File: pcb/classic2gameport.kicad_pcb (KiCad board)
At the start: 2 copper layers, 58 x 45 mm, 39 parts, among them J1 Conn_01x04, J2 Conn_02x05_Odd_Even, J3 DB15_Male, J4 Conn_01x04, Q1 Q_PMOS_GSD, Q2 Q_PMOS_GSD, Q3 Q_PMOS_GSD, Q4 Q_PMOS_GSD, Q5 Q_PMOS_GSD, Q6 Q_PMOS_GSD, Q7 Q_PMOS_GSD, Q8 Q_PMOS_GSD, U1 74HC14, U2 74HC14, U3 LM3480-3.3, U4 STM32F030K6Tx

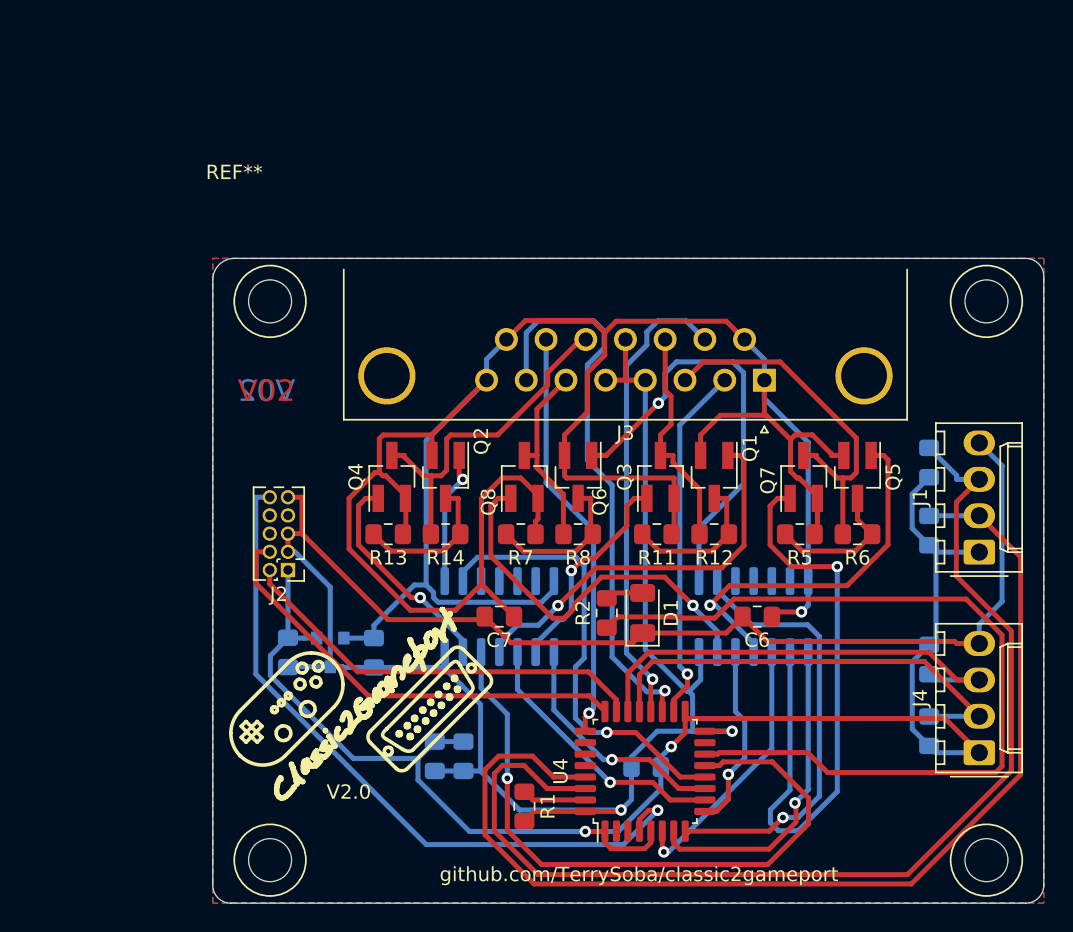
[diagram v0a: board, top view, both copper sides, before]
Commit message: Redesign again
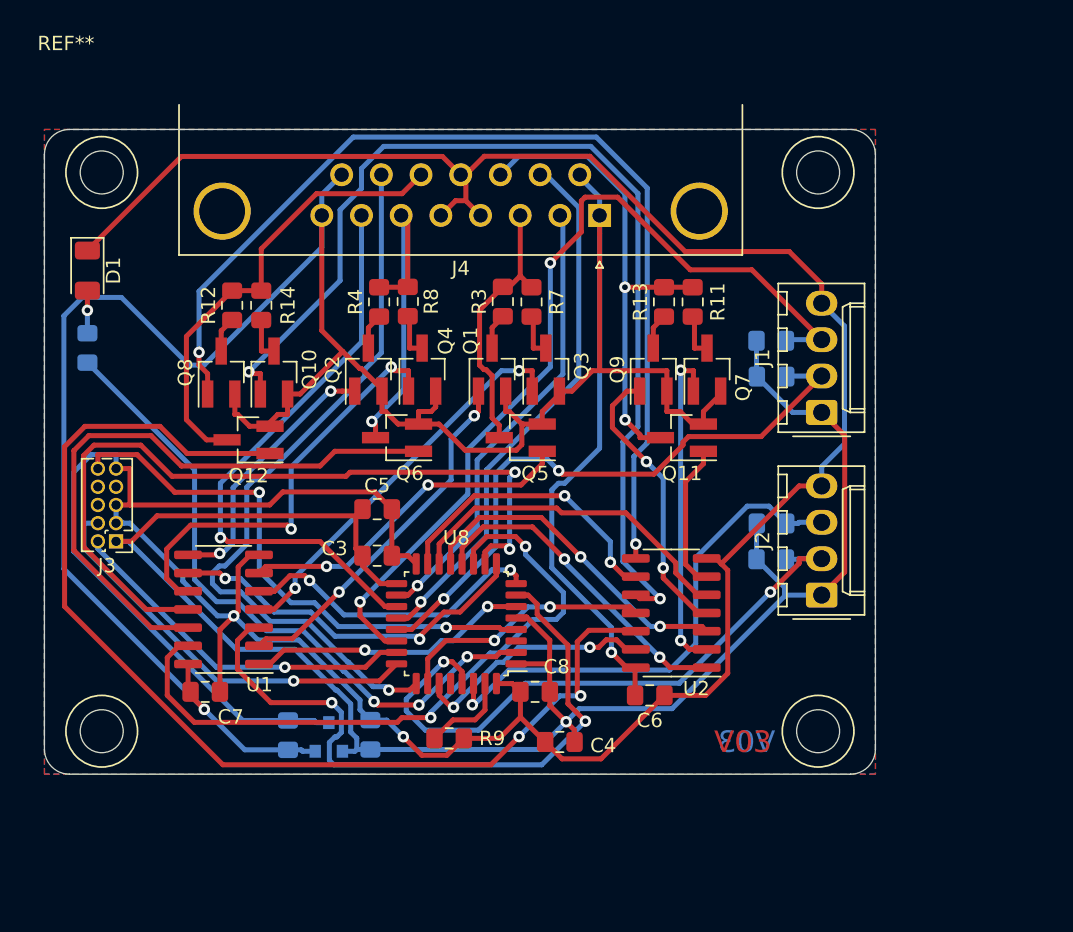
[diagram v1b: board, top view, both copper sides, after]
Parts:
- removed U3: LM3480-3.3, Package_TO_SOT_SMD:SOT-23
- removed U4: STM32F030K6Tx, Package_QFP:LQFP-32_7x7mm_P0.8mm
- added C8: 100nF, Capacitor_SMD:C_0805_2012Metric_Pad1.15x1.40mm_HandSolder, F.Cu at (107.0, 67.8)
- added Q10: Q_PMOS_GSD, Package_TO_SOT_SMD:SOT-23_Handsoldering, F.Cu at (88.8, 45.5)
- added Q11: Q_PMOS_GSD, Package_TO_SOT_SMD:SOT-23_Handsoldering, F.Cu at (117.2, 50.0)
- added Q12: Q_PMOS_GSD, Package_TO_SOT_SMD:SOT-23_Handsoldering, F.Cu at (87.0, 50.2)
- added Q9: Q_PMOS_GSD, Package_TO_SOT_SMD:SOT-23_Handsoldering, F.Cu at (115.2, 45.3)
- added U5: LM3480-3.3, Package_TO_SOT_SMD:SOT-23, B.Cu at (92.6, 70.9)
- added U8: STM32F030K6Tx, Package_QFP:LQFP-32_7x7mm_P0.8mm, F.Cu at (101.5, 63.0)
- C3: value 1µF -> 100nF; moved to F.Cu
- C4: value 4.7µF -> 1µF; moved to F.Cu
- C5: value 100nF -> 4.7µF; moved to F.Cu
- J2: value Conn_02x05_Odd_Even -> Conn_01x04; footprint Connector_PinHeader_1.27mm:PinHeader_2x05_P1.27mm_Vertical -> Connector_Molex:Molex_KK-254_AE-6410-04A_1x04_P2.54mm_Vertical
- J3: value DB15_Male -> Conn_02x05_Odd_Even; footprint Connector_Dsub:DSUB-15_Male_Horizontal_P2.77x2.84mm_EdgePinOffset4.94mm_Housed_MountingHolesOffset7.48mm -> Connector_PinHeader_1.27mm:PinHeader_2x05_P1.27mm_Vertical
- J4: value Conn_01x04 -> DB15_Male; footprint Connector_Molex:Molex_KK-254_AE-6410-04A_1x04_P2.54mm_Vertical -> Connector_Dsub:DSUB-15_Male_Horizontal_P2.77x2.84mm_EdgePinOffset4.94mm_Housed_MountingHolesOffset7.48mm
- R1: value 10k -> 1kR; moved to B.Cu
- R10: value 1kR -> 470R
- R11, R12, R13, R14, R7, R8: value 49k9 -> 100kR
- R2: value 470R -> 1kR; moved to B.Cu
- R3, R4: value 1kR -> 100kR; moved to F.Cu
- R5, R6: value 49k9 -> 1kR; moved to B.Cu
- R9: value 1kR -> 10k; moved to F.Cu
- U1, U2: moved to F.Cu
- moved R10 62.6 mm to (75.8, 43.8), turned to 90 degrees
- moved J3 46.6 mm to (77.8, 57.2)
- moved J4 45.9 mm to (111.5, 34.5), turned to 180 degrees
- moved D1 45.5 mm to (75.8, 38.4), turned to 270 degrees
- moved R4 40.0 mm to (96.1, 40.5)
- moved J2 37.3 mm to (127.0, 61.0), turned to 90 degrees
- moved R12 37.2 mm to (85.9, 40.8), turned to 90 degrees
- moved U1 37.0 mm to (85.2, 62.0), turned to 180 degrees
- moved R1 34.6 mm to (123.5, 45.8), turned to 0 degrees
- moved R3 33.8 mm to (104.7, 40.5)
- moved R9 33.5 mm to (101.0, 71.0), turned to 0 degrees
- moved C5 26.0 mm to (96.0, 55.0), turned to 0 degrees
- moved R13 25.2 mm to (116.0, 40.5), turned to 90 degrees
- moved Q5 23.7 mm to (106.0, 50.0), turned to 180 degrees
- moved Q8 22.4 mm to (85.1, 45.5)
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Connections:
- C1 pad 1: 5V -> 3.3V
- C2 pad 1: 3.3V -> 5V
- J1 pad 2: SCL -> SCL2
- J1 pad 3: SDA -> SDA2
- J2 pad 2: SWDIO -> SCL
- J2 pad 3: GND -> SDA
- J2 pad 4: SWCLK -> GND
- J3 pad 1: 5V -> 3.3V
- J3 pad 10: BUTTON3 -> NRST
- J3 pad 2: BUTTON1 -> SWDIO
- J3 pad 3: JS1_X_AXIS -> GND
- J3 pad 4: GND -> SWCLK
- J3 pad 6: JS1_Y_AXIS -> (no net)
- J3 pad 7: BUTTON2 -> (no net)
- J3 pad 8: 5V -> (no net)
- J3 pad 9: 5V -> GND
- J4 pad 1: 3.3V -> 5V
- J4 pad 2: SCL2 -> BUTTON1
- J4 pad 3: SDA2 -> JS1_X_AXIS
- Q3 pad 3: JS2_X_AXIS -> Net-(Q3-Pad3)
- Q4 pad 3: JS2_Y_AXIS -> Net-(Q4-Pad3)
- Q5 pad 3: Net-(Q5-Pad3) -> JS1_X_AXIS
- Q6 pad 3: Net-(Q6-Pad3) -> JS1_Y_AXIS
- Q7 pad 3: JS1_X_AXIS -> Net-(Q7-Pad3)
- Q8 pad 3: JS1_Y_AXIS -> Net-(Q8-Pad3)
- R1 pad 1: Net-(R1-Pad1) -> 3.3V
- R1 pad 2: GND -> SCL2
- R10 pad 1: 3.3V -> Net-(R10-Pad1)
- R10 pad 2: SDA2 -> Net-(D1-Pad2)
- R11 pad 1: 5V -> Net-(Q7-Pad3)
- R11 pad 2: Net-(Q1-Pad3) -> JS2_X_AXIS
- R12 pad 1: Net-(Q1-Pad3) -> Net-(Q8-Pad3)
- R12 pad 2: JS2_X_AXIS -> JS2_Y_AXIS
- R13 pad 1: 5V -> Net-(Q9-Pad3)
- R13 pad 2: Net-(Q2-Pad3) -> JS2_X_AXIS
- R14 pad 1: Net-(Q2-Pad3) -> Net-(Q10-Pad3)
- R2 pad 1: Net-(R2-Pad1) -> 3.3V
- R2 pad 2: Net-(D1-Pad2) -> SCL
- R3 pad 1: 3.3V -> Net-(Q1-Pad3)
- R3 pad 2: SCL -> JS1_X_AXIS
- R4 pad 1: 3.3V -> Net-(Q2-Pad3)
- R4 pad 2: SDA -> JS1_Y_AXIS
- R5 pad 1: 5V -> 3.3V
- R5 pad 2: Net-(Q5-Pad3) -> SDA2
- R6 pad 1: Net-(Q5-Pad3) -> 3.3V
- R6 pad 2: JS1_X_AXIS -> SDA
- R7 pad 1: 5V -> Net-(Q3-Pad3)
- R7 pad 2: Net-(Q6-Pad3) -> JS1_X_AXIS
- R8 pad 1: Net-(Q6-Pad3) -> Net-(Q4-Pad3)
- R9 pad 1: 3.3V -> Net-(R9-Pad1)
- R9 pad 2: SCL2 -> GND
- U1 pad 1: JS1_X2 -> JS1_X1
- U1 pad 10: (no net) -> Net-(Q4-Pad1)
- U1 pad 11: (no net) -> JS1_Y2
- U1 pad 12: (no net) -> Net-(Q6-Pad1)
- U1 pad 13: (no net) -> JS1_Y3
- U1 pad 2: Net-(Q7-Pad1) -> Net-(Q1-Pad1)
- U1 pad 3: JS1_X1 -> JS1_X2
- U1 pad 4: Net-(Q5-Pad1) -> Net-(Q3-Pad1)
- U1 pad 5: JS1_Y2 -> JS1_X3
- U1 pad 6: Net-(Q8-Pad1) -> Net-(Q5-Pad1)
- U1 pad 8: Net-(Q6-Pad1) -> Net-(Q2-Pad1)
- U2 pad 1: JS2_X2 -> JS2_X1
- U2 pad 10: (no net) -> Net-(Q10-Pad1)
- U2 pad 11: (no net) -> JS2_Y2
- U2 pad 12: (no net) -> Net-(Q12-Pad1)
- U2 pad 13: (no net) -> JS2_Y3
- U2 pad 2: Net-(Q3-Pad1) -> Net-(Q7-Pad1)
- U2 pad 3: JS2_X1 -> JS2_X2
- U2 pad 4: Net-(Q1-Pad1) -> Net-(Q9-Pad1)
- U2 pad 5: JS2_Y2 -> JS2_X3
- U2 pad 6: Net-(Q4-Pad1) -> Net-(Q11-Pad1)
- U2 pad 8: Net-(Q2-Pad1) -> Net-(Q8-Pad1)
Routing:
- net Net-(Q12-Pad1): track 0.00 -> 77.8 mm, vias 0 -> 2
- net Net-(Q10-Pad1): track 0.00 -> 72.6 mm, vias 0 -> 2
- net Net-(R2-Pad1): track 60.2 -> 0.00 mm
- net GND: track 172.6 -> 230.5 mm
- net JS1_Y3: track 0.00 -> 47.2 mm, vias 0 -> 2
- net Net-(R10-Pad1): track 0.00 -> 45.9 mm, vias 0 -> 3
- net Net-(Q8-Pad1): track 27.1 -> 70.9 mm, vias 1 -> 2
- net SDA: track 78.8 -> 35.7 mm, vias 0 -> 1
- net JS1_Y2: track 13.0 -> 55.3 mm, vias 1 -> 2
- net SCL: track 77.3 -> 44.1 mm, vias 0 -> 2
- net SDA2: track 32.3 -> 62.2 mm, vias 0 -> 2
- net JS2_Y2: track 46.6 -> 17.9 mm, vias 1 -> 2
- net JS1_X2: track 22.6 -> 46.7 mm, vias 1 -> 2
- net JS2_X3: track 0.00 -> 24.0 mm
- net BUTTON4: track 29.0 -> 51.4 mm
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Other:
- outline, holes or cut-outs redrawn
- board text added: "V03"
- board text added: "V3.0"
- board text removed: "V02"
- board text removed: "V2.0"
